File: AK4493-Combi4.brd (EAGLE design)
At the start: 178 x 151.3 mm, 226 parts, among them IC1 LT3042, IC3 AK4493, IC4 LT3042, IC4A SN74ABT273DBR, IC5 LT3042, IC6 LT3042, IC7 LT3042, IC8 LT3042, IC9 AK4493, J15 XR2A-0811-N, J16 XR2A-0811-N, J17 XR2A-0811-N, J18 XR2A-0811-N, J19 XR2A-0811-N, J20 XR2A-0811-N, J26 SJ-63033A, J27 1935161, U1 AZ1117H-5.0TRE1, X1 JST-XH-07-PIN-ROUND-PAD, X4 JST-XH-04-PIN-ROUND-PAD

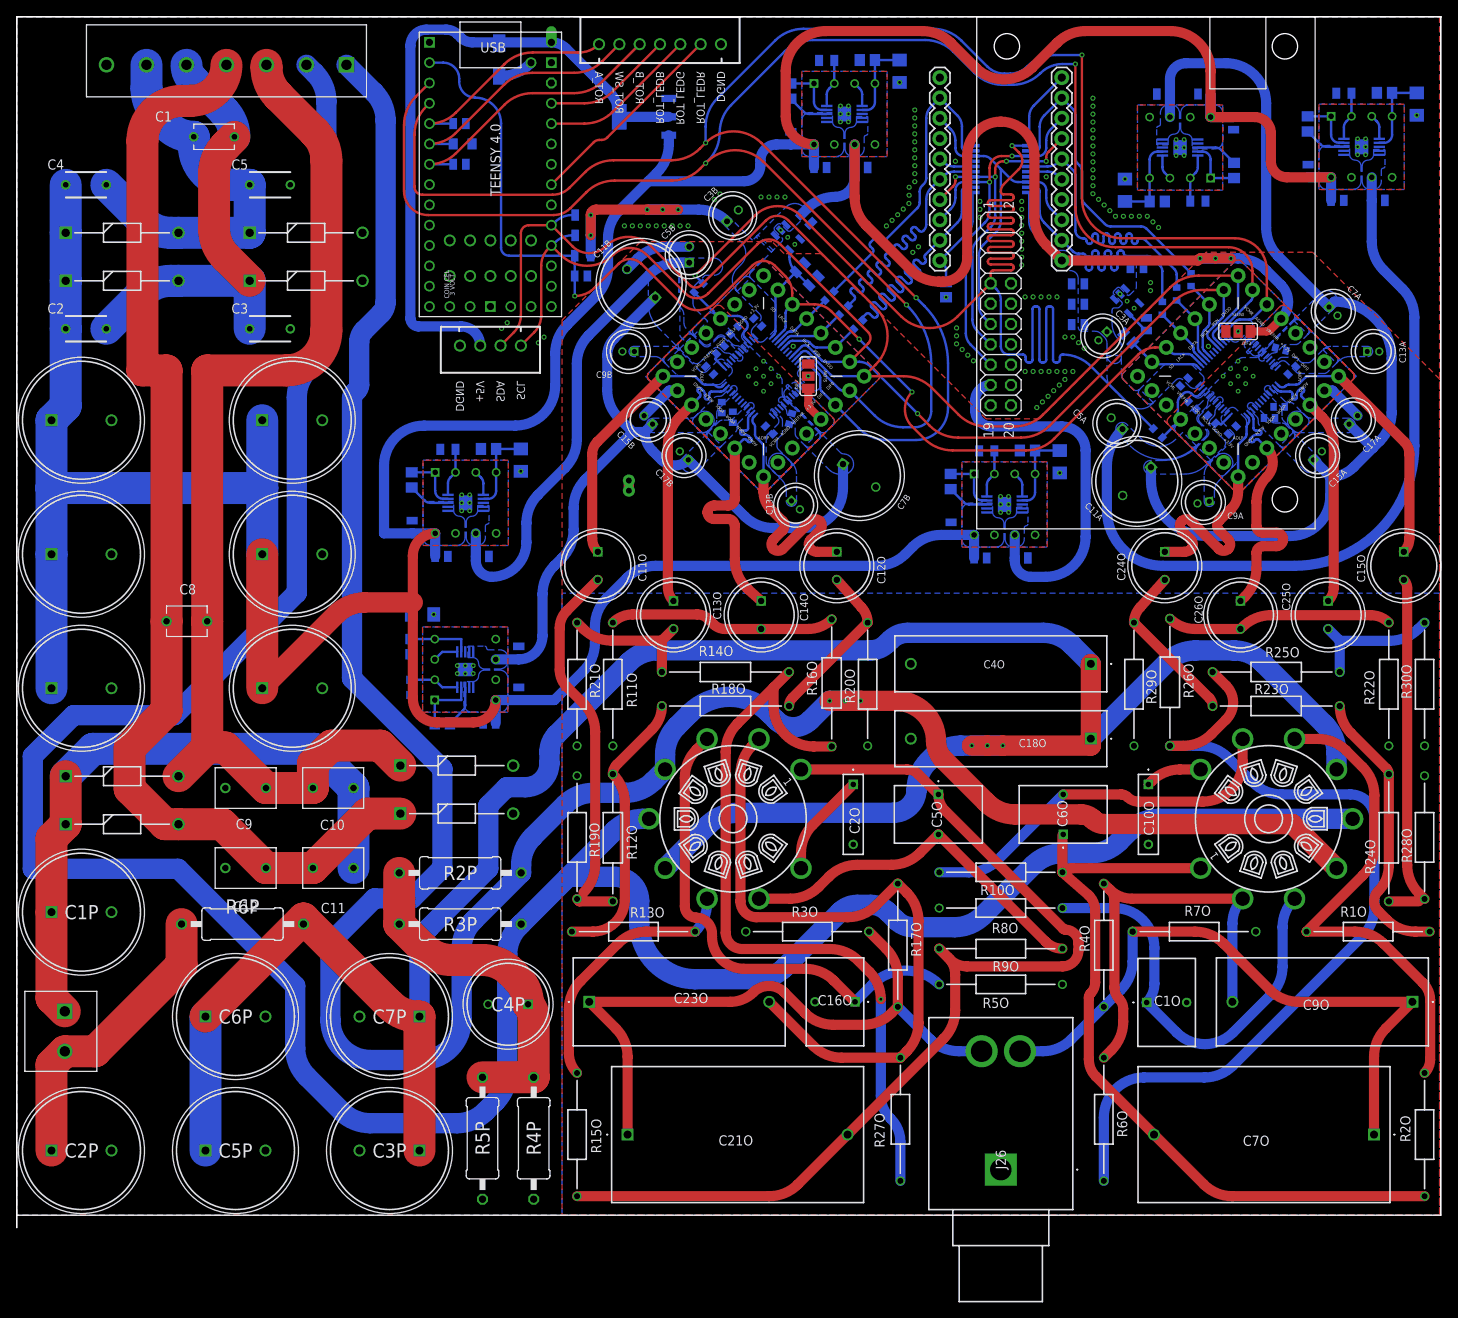
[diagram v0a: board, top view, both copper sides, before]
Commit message: Progress
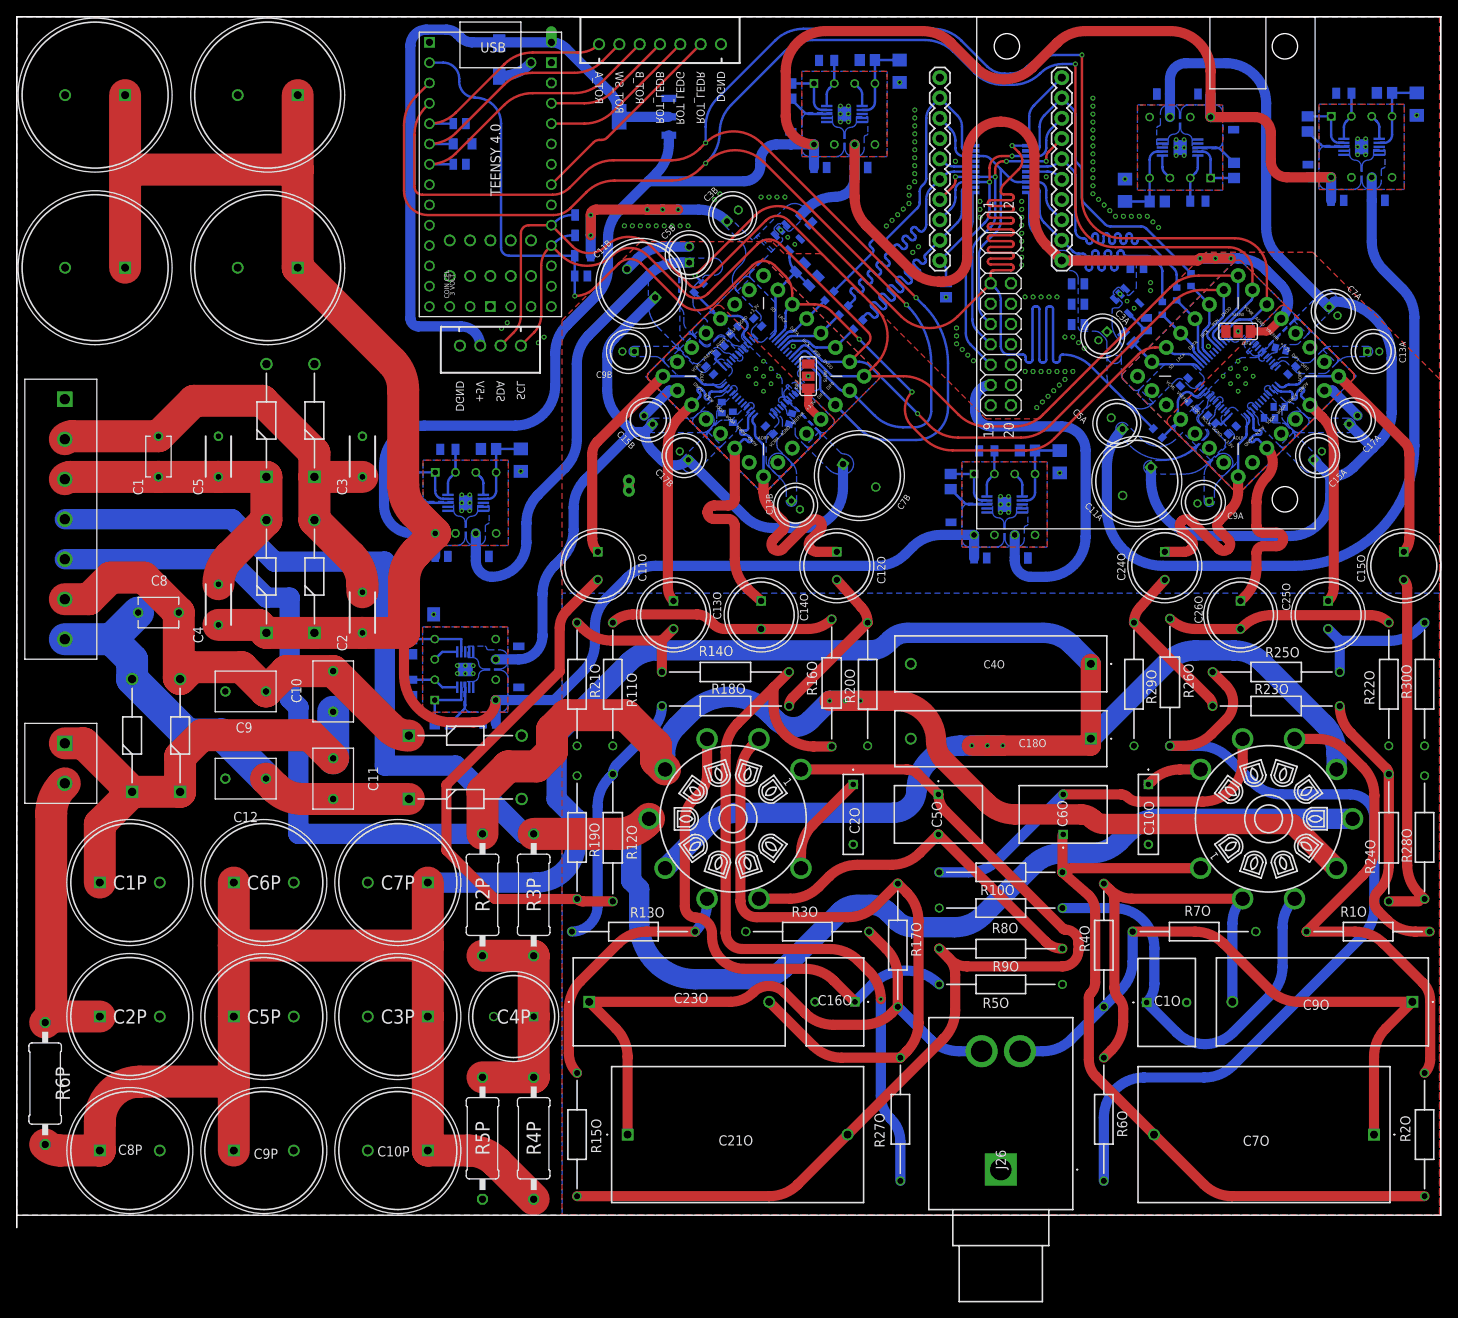
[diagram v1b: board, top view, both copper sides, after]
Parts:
- removed C6P1, C7P1: 68u, Dual Mono Amp Library:CAPPRD750W80D1475H4700
- added C10P, C8P, C9P: 68u, Dual Mono Amp Library:CAPPRD750W80D1475H4700
- C1P1, C2P1, C3P1, C5P1: device Dual Mono Amp Library:CAPPRD750W80D1475H4700 -> Dual Mono Amp Library:CAPPRD750W80D1825H3750
- moved C3P1 65.1 mm to (35.1, 140.0), turned to 180 degrees
- moved C5P1 59.9 mm to (13.5, 140.0), turned to 180 degrees
- moved D8 56.0 mm to (31.2, 72.8), turned to 90 degrees
- moved C4 55.0 mm to (25.2, 76.3), turned to 90 degrees
- moved IN 54.7 mm to (6.00, 102.0), turned to 270 degrees
- moved D7 53.9 mm to (37.2, 72.8), turned to 90 degrees
- moved C2 49.5 mm to (43.2, 75.3), turned to 90 degrees
- moved C1 40.2 mm to (17.7, 94.8), turned to 90 degrees
- moved C1P1 36.2 mm to (35.1, 118.4), turned to 180 degrees
- moved C5 34.6 mm to (25.2, 94.8), turned to 90 degrees
- moved J27 33.5 mm to (6.00, 59.0)
- moved R6P 31.7 mm to (3.54, 16.5), turned to 90 degrees
- moved D5 30.6 mm to (31.2, 92.3), turned to 90 degrees
- moved D6 25.8 mm to (37.2, 92.3), turned to 90 degrees
- moved C2P1 25.6 mm to (13.5, 118.4), turned to 180 degrees
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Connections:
- removed net VCC/1: C1P1.1, C2.1, C20A.1, C20B.1, C20C.1, C20D.1, C20E.1, C20F.1, C21A.1, C21B.1, C21C.1, C21D.1, C21E.1, C21F.1, C2P1.1, C3P1.1, C4.1, C5P1.1, C6P1.1, C7P1.1, D7.1, D8.1, IC1.1, IC1.2, IC1.3, IC4.1, IC4.2, IC4.3, IC5.1, IC5.2, IC5.3, IC6.1, IC6.2, IC6.3, IC7.1, IC7.2, IC7.3, IC8.1, IC8.2, IC8.3, J15.7, J15.8, J16.7, J16.8, J17.7, J17.8, J18.7, J18.8, J19.7, J19.8, J20.7, J20.8, R8A.1, R8B.1, R8C.1, R8D.1, R8E.1, R8F.1, U1.3
- net +240VDC: now also C10P.1, C8P.1, C9P.1, R4P.2
- net 115_VAC_BLK: now also IN.7; no longer IN.4
- net 115_VAC_RED: now also IN.6; no longer IN.3
- net 6.3_VAC_BLU: now also IN.2; no longer IN.5
- net 6.3_VAC_GRN: now also IN.3; no longer IN.6
- net 66.3VAC/1: now also IN.5; no longer IN.1
- net 66.3VAC/2: now also IN.4; no longer IN.2
- net DGND: now also C10P.2, C8P.2, C9P.2; no longer C6P1.2, C7P1.2
- net PE: now also IN.1; no longer IN.7
- net VCC: now also C1P1.1, C2.1, C20A.1, C20B.1, C20C.1, C20D.1, C20E.1, C20F.1, C21A.1, C21B.1, C21C.1, C21D.1, C21E.1, C21F.1, C2P1.1, C3P1.1, C4.1, C5P1.1, D7.1, D8.1, IC1.1, IC1.2, IC1.3, IC4.1, IC4.2, IC4.3, IC5.1, IC5.2, IC5.3, IC6.1, IC6.2, IC6.3, IC7.1, IC7.2, IC7.3, IC8.1, IC8.2, IC8.3, J15.7, J15.8, J16.7, J16.8, J17.7, J17.8, J18.7, J18.8, J19.7, J19.8, J20.7, J20.8, R8A.1, R8B.1, R8C.1, R8D.1, R8E.1, R8F.1, U1.3; no longer R4P.2
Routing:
- net VCC/1: track 502.3 -> 0.00 mm
- net VCC: track 0.00 -> 481.3 mm
- net 66.3VAC/2: track 357.6 -> 219.7 mm
- net 115_VAC_BLK: track 141.1 -> 57.1 mm
- net 66.3VAC/1: track 304.4 -> 223.4 mm
- net 115_VAC_RED: track 136.1 -> 60.2 mm
- net +240VDC: track 303.5 -> 360.7 mm
- net N$64: track 80.2 -> 61.6 mm
- net N$33: track 48.2 -> 64.8 mm
- net N$67: track 42.5 -> 28.0 mm
- net 6.3_VAC_GRN: track 48.1 -> 40.9 mm
- net 6.3_VAC_BLU: track 57.4 -> 61.4 mm
- net R+: track 35.0 -> 32.2 mm
- net N$65: track 37.3 -> 36.7 mm
- added copper zone on layer 16, net VCC
- removed copper zone on layer 16, net VCC/1
